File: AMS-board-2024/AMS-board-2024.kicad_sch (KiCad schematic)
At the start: 66 parts, among them J1 XH_6pin_SMT, J10 XH_6pin_SMT, J11 XH_3pin_SMT, J12 XH_4pin_SMT, J13 XH_6pin_SMT, J14 XH_3pin_SMT, J15 XH_4pin_SMT, J16 XH_6pin_SMT, J17 XH_3pin_SMT, J18 XH_4pin_SMT, J19 19427-0040, J2 XH_3pin_SMT, J20 19427-0040, J21 XH_6pin_SMT, J22 XH_3pin_SMT, J23 XH_4pin_SMT, J24 XH_6pin_SMT, J25 XH_3pin_SMT, J26 XH_4pin_SMT, J27 XH_2pin_Side, J28 XH_6pin_Side, J29 XH_5pin_Side, J3 XH_4pin_SMT, J30 PinHeader_02x05_P1.00mm, J31 XH_2pin_Side, J32 5077CR-16-SMC2-BK-TR, J33 XH_5pin_Side, J34 XH_6pin_SMT, J35 XH_6pin_SMT, J36 XH_6pin_SMT, J37 XH_6pin_SMT, J38 XH_6pin_SMT, J39 XH_6pin_SMT, J4 XH_6pin_SMT, J40 XH_6pin_SMT, J41 XH_6pin_SMT, J5 XH_3pin_SMT, J6 XH_4pin_SMT, J7 XH_6pin_SMT, J8 XH_3pin_SMT, J9 XH_4pin_SMT

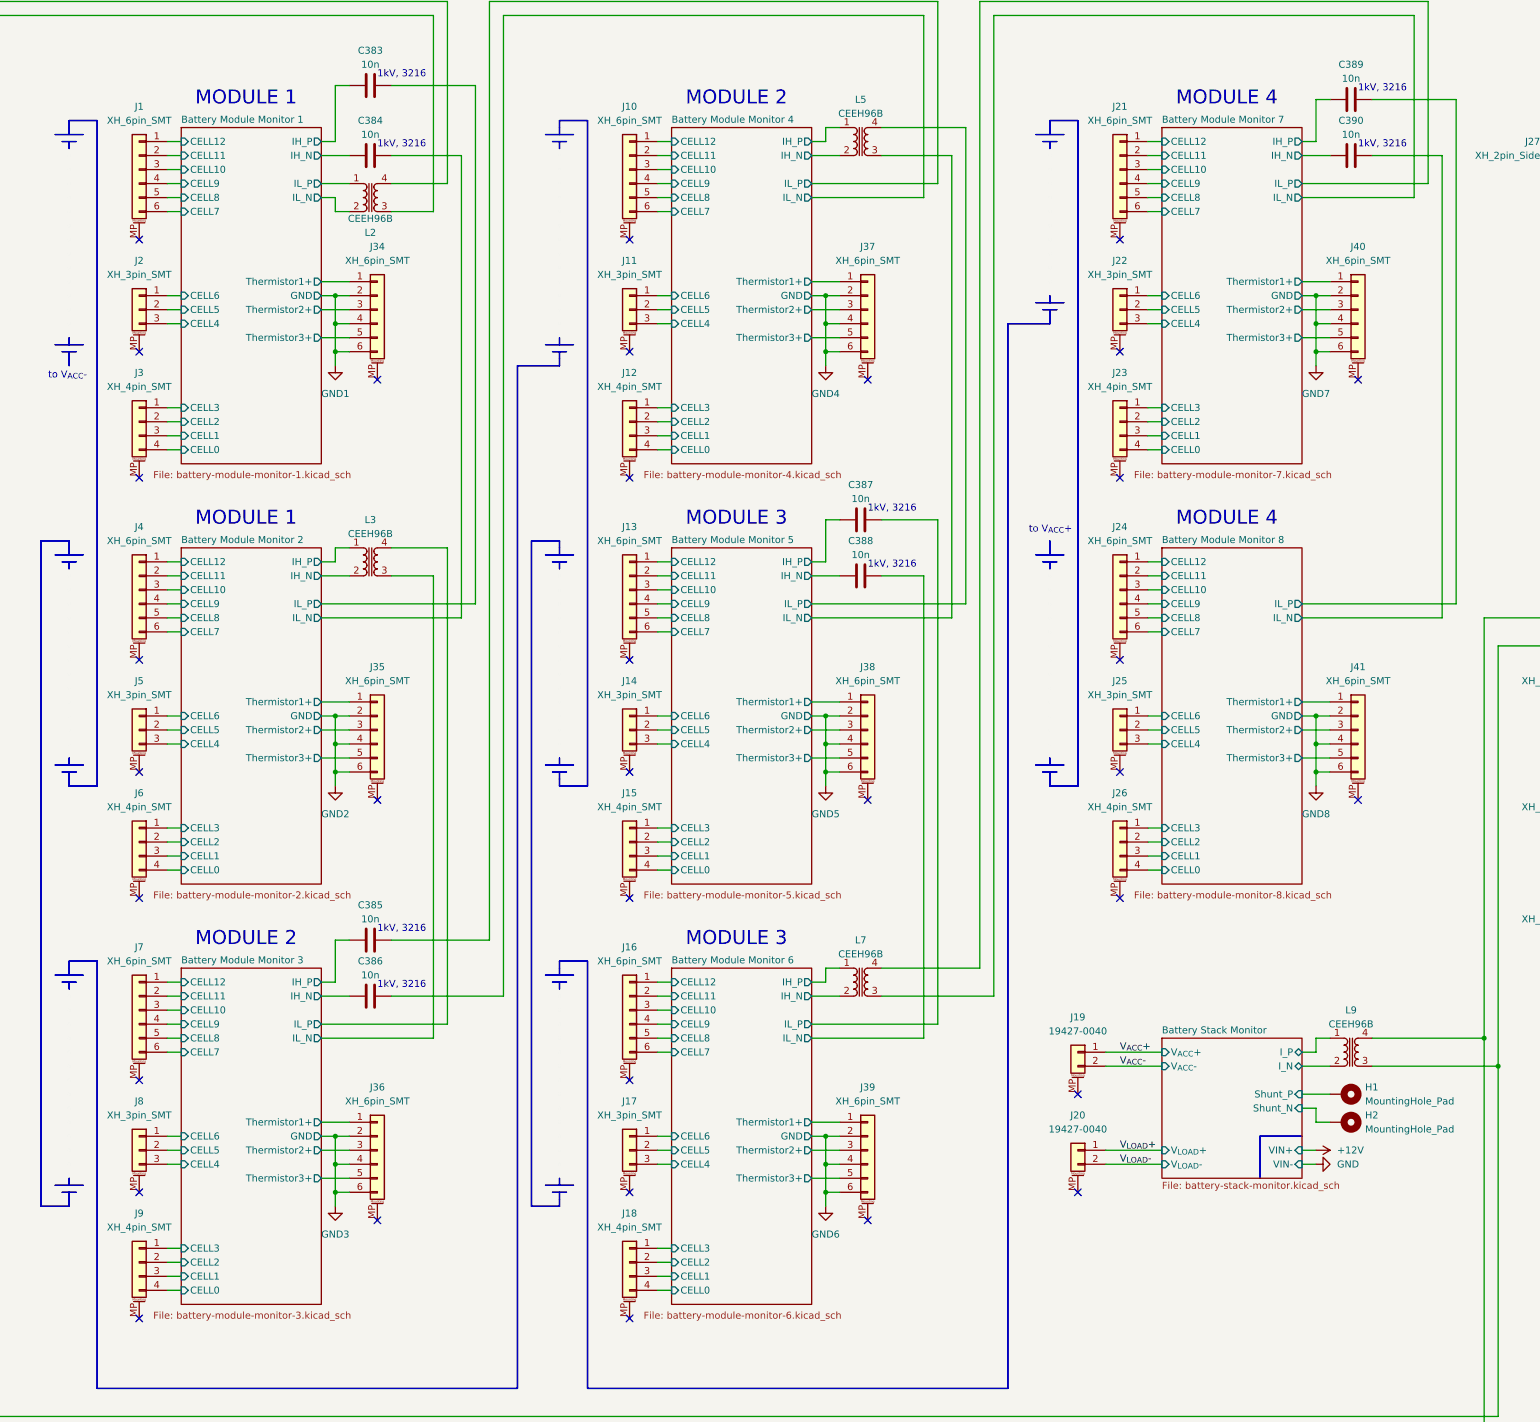
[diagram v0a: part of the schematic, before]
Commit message: セル監視コネクタを34691-0200に変更
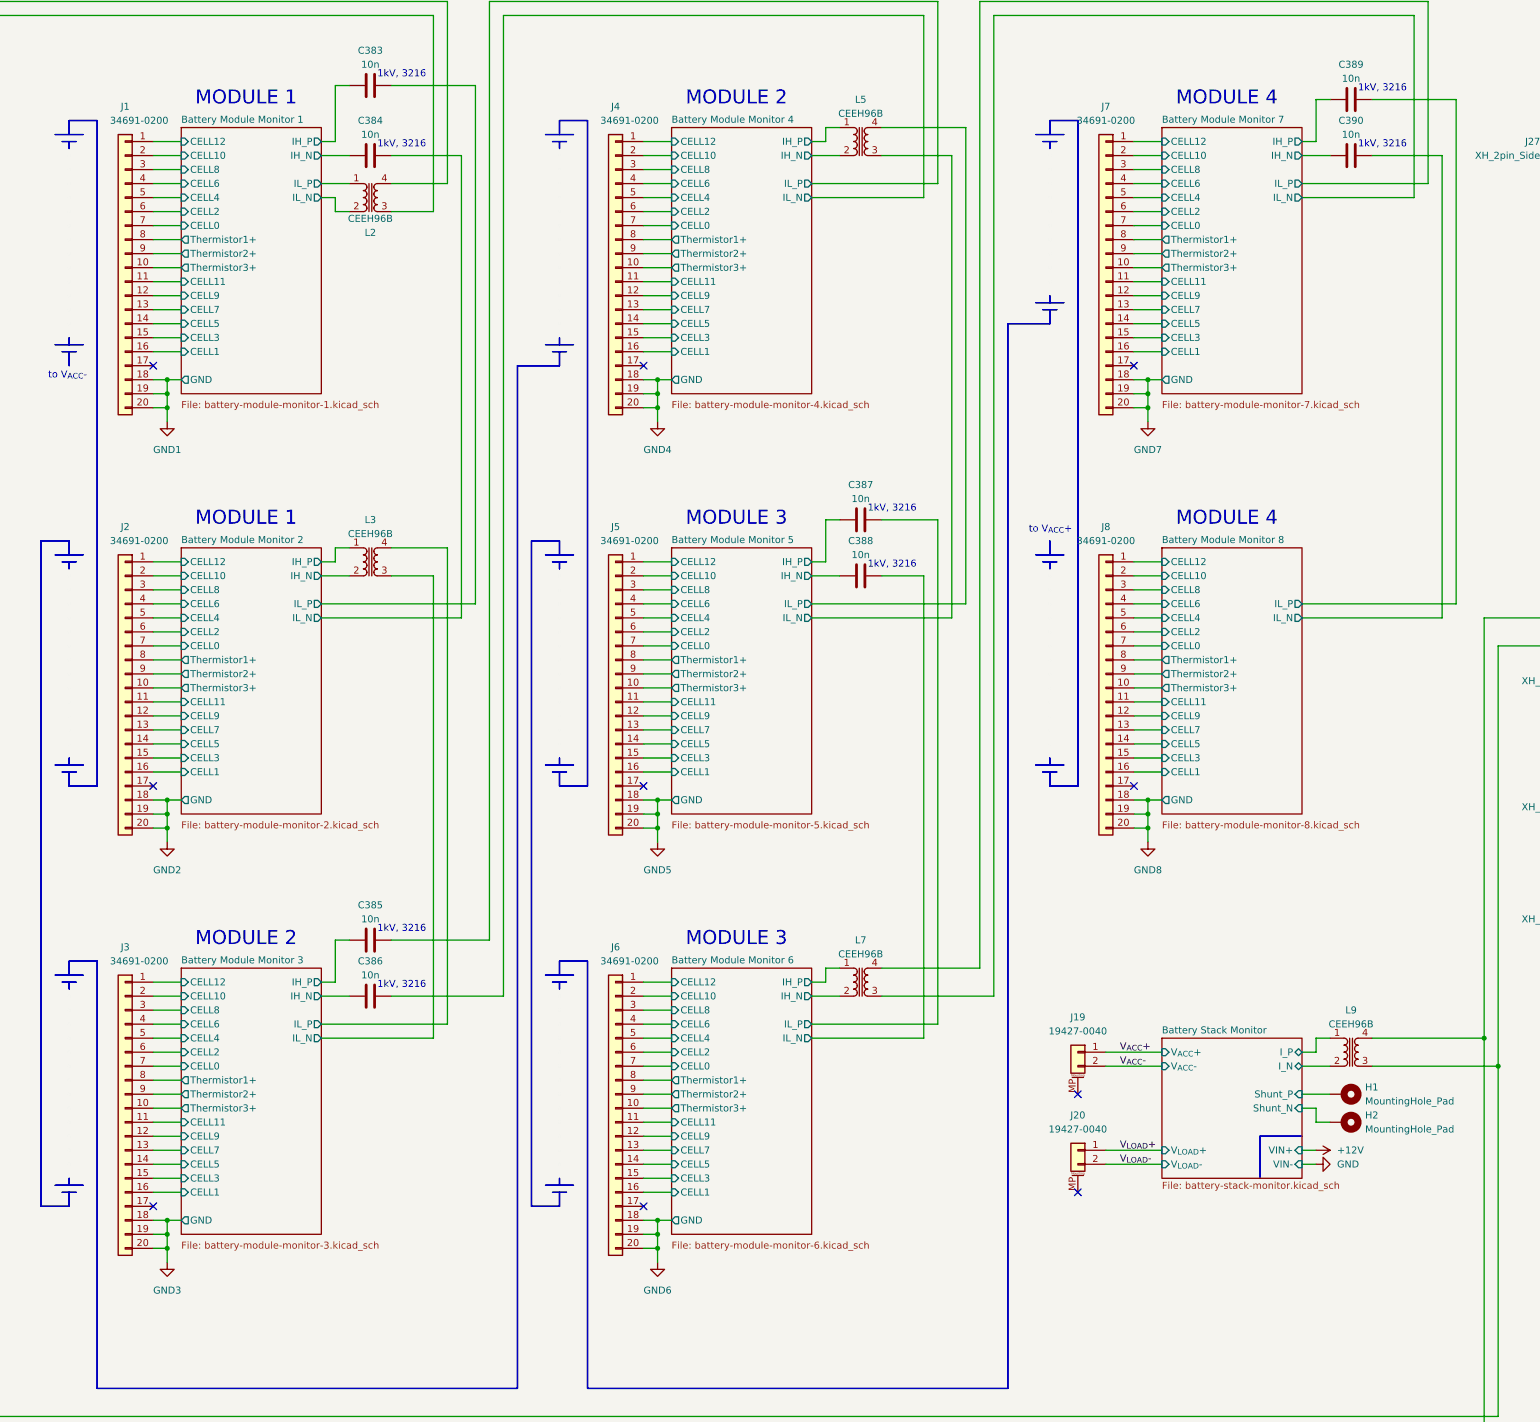
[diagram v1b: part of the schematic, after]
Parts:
- removed J1, J10, J13, J16, J21, J24, J34, J35, J36, J37, J38, J39, J4, J40, J41, J7: XH_6pin_SMT, ProjectEV:Connector_S6B-XH-SM4-TB, symbol ProjectEV:Connector_XH_6pin_SMT
- removed J11, J14, J17, J2, J22, J25, J5, J8: XH_3pin_SMT, ProjectEV:Connector_S3B-XH-SM4-TB, symbol ProjectEV:Connector_XH_3pin_SMT
- removed J12, J15, J18, J23, J26, J3, J6, J9: XH_4pin_SMT, ProjectEV:Connector_S4B-XH-SM4-TB, symbol ProjectEV:Connector_XH_4pin_SMT
- added J1, J2, J3, J4, J5, J6, J7, J8: 34691-0200, ProjectEV:Connector_34691-0200, symbol ProjectEV:Connector_34691-0200
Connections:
- net Battery Module Monitor 1/CELL0: now also J1.7 (Pin_7)
- net Battery Module Monitor 1/CELL1: now also J1.16 (Pin_16)
- net Battery Module Monitor 1/CELL10: now also J1.2 (Pin_2)
- net Battery Module Monitor 1/CELL11: now also J1.11 (Pin_11)
- net Battery Module Monitor 1/CELL12: now also J1.1 (Pin_1)
- net Battery Module Monitor 1/CELL2: now also J1.6 (Pin_6)
- net Battery Module Monitor 1/CELL3: now also J1.15 (Pin_15)
- net Battery Module Monitor 1/CELL4: now also J1.5 (Pin_5)
- net Battery Module Monitor 1/CELL5: now also J1.14 (Pin_14)
- net Battery Module Monitor 1/CELL6: now also J1.4 (Pin_4)
- net Battery Module Monitor 1/CELL7: now also J1.13 (Pin_13)
- net Battery Module Monitor 1/CELL8: now also J1.3 (Pin_3)
- net Battery Module Monitor 1/CELL9: now also J1.12 (Pin_12)
- net Battery Module Monitor 1/Thermistor1+: now also J1.8 (Pin_8)
- net Battery Module Monitor 1/Thermistor2+: now also J1.9 (Pin_9)
- net Battery Module Monitor 1/Thermistor3+: now also J1.10 (Pin_10)
- net Battery Module Monitor 2/CELL0: now also J2.7 (Pin_7)
- net Battery Module Monitor 2/CELL1: now also J2.16 (Pin_16)
- net Battery Module Monitor 2/CELL10: now also J2.2 (Pin_2)
- net Battery Module Monitor 2/CELL11: now also J2.11 (Pin_11)
- net Battery Module Monitor 2/CELL12: now also J2.1 (Pin_1)
- net Battery Module Monitor 2/CELL2: now also J2.6 (Pin_6)
- net Battery Module Monitor 2/CELL3: now also J2.15 (Pin_15)
- net Battery Module Monitor 2/CELL4: now also J2.5 (Pin_5)
- net Battery Module Monitor 2/CELL5: now also J2.14 (Pin_14)
- net Battery Module Monitor 2/CELL6: now also J2.4 (Pin_4)
- net Battery Module Monitor 2/CELL7: now also J2.13 (Pin_13)
- net Battery Module Monitor 2/CELL8: now also J2.3 (Pin_3)
- net Battery Module Monitor 2/CELL9: now also J2.12 (Pin_12)
- net Battery Module Monitor 2/Thermistor1+: now also J2.8 (Pin_8)
- net Battery Module Monitor 2/Thermistor2+: now also J2.9 (Pin_9)
- net Battery Module Monitor 2/Thermistor3+: now also J2.10 (Pin_10)
- net Battery Module Monitor 3/CELL0: now also J3.7 (Pin_7)
- net Battery Module Monitor 3/CELL1: now also J3.16 (Pin_16)
- net Battery Module Monitor 3/CELL10: now also J3.2 (Pin_2)
- net Battery Module Monitor 3/CELL11: now also J3.11 (Pin_11)
- net Battery Module Monitor 3/CELL12: now also J3.1 (Pin_1)
- net Battery Module Monitor 3/CELL2: now also J3.6 (Pin_6)
- net Battery Module Monitor 3/CELL3: now also J3.15 (Pin_15)
- net Battery Module Monitor 3/CELL4: now also J3.5 (Pin_5)
- net Battery Module Monitor 3/CELL5: now also J3.14 (Pin_14)
- net Battery Module Monitor 3/CELL6: now also J3.4 (Pin_4)
- net Battery Module Monitor 3/CELL7: now also J3.13 (Pin_13)
- net Battery Module Monitor 3/CELL8: now also J3.3 (Pin_3)
- net Battery Module Monitor 3/CELL9: now also J3.12 (Pin_12)
- net Battery Module Monitor 3/Thermistor1+: now also J3.8 (Pin_8)
- net Battery Module Monitor 3/Thermistor2+: now also J3.9 (Pin_9)
- net Battery Module Monitor 3/Thermistor3+: now also J3.10 (Pin_10)
- net Battery Module Monitor 4/CELL0: now also J4.7 (Pin_7)
- net Battery Module Monitor 4/CELL1: now also J4.16 (Pin_16)
- net Battery Module Monitor 4/CELL10: now also J4.2 (Pin_2)
- net Battery Module Monitor 4/CELL11: now also J4.11 (Pin_11)
- net Battery Module Monitor 4/CELL12: now also J4.1 (Pin_1)
- net Battery Module Monitor 4/CELL2: now also J4.6 (Pin_6)
- net Battery Module Monitor 4/CELL3: now also J4.15 (Pin_15)
- net Battery Module Monitor 4/CELL4: now also J4.5 (Pin_5)
- net Battery Module Monitor 4/CELL5: now also J4.14 (Pin_14)
- net Battery Module Monitor 4/CELL6: now also J4.4 (Pin_4)
- net Battery Module Monitor 4/CELL7: now also J4.13 (Pin_13)
- net Battery Module Monitor 4/CELL8: now also J4.3 (Pin_3)
- net Battery Module Monitor 4/CELL9: now also J4.12 (Pin_12)
- net Battery Module Monitor 4/Thermistor1+: now also J4.8 (Pin_8)
- net Battery Module Monitor 4/Thermistor2+: now also J4.9 (Pin_9)
- net Battery Module Monitor 4/Thermistor3+: now also J4.10 (Pin_10)
- net Battery Module Monitor 5/CELL0: now also J5.7 (Pin_7)
- net Battery Module Monitor 5/CELL1: now also J5.16 (Pin_16)
- net Battery Module Monitor 5/CELL10: now also J5.2 (Pin_2)
- net Battery Module Monitor 5/CELL11: now also J5.11 (Pin_11)
- net Battery Module Monitor 5/CELL12: now also J5.1 (Pin_1)
- net Battery Module Monitor 5/CELL2: now also J5.6 (Pin_6)
- net Battery Module Monitor 5/CELL3: now also J5.15 (Pin_15)
- net Battery Module Monitor 5/CELL4: now also J5.5 (Pin_5)
- net Battery Module Monitor 5/CELL5: now also J5.14 (Pin_14)
- net Battery Module Monitor 5/CELL6: now also J5.4 (Pin_4)
- net Battery Module Monitor 5/CELL7: now also J5.13 (Pin_13)
- net Battery Module Monitor 5/CELL8: now also J5.3 (Pin_3)
- net Battery Module Monitor 5/CELL9: now also J5.12 (Pin_12)
- net Battery Module Monitor 5/Thermistor1+: now also J5.8 (Pin_8)
- net Battery Module Monitor 5/Thermistor2+: now also J5.9 (Pin_9)
- net Battery Module Monitor 5/Thermistor3+: now also J5.10 (Pin_10)
- net Battery Module Monitor 6/CELL0: now also J6.7 (Pin_7)
- net Battery Module Monitor 6/CELL1: now also J6.16 (Pin_16)
- net Battery Module Monitor 6/CELL10: now also J6.2 (Pin_2)
- net Battery Module Monitor 6/CELL11: now also J6.11 (Pin_11)
- net Battery Module Monitor 6/CELL12: now also J6.1 (Pin_1)
- net Battery Module Monitor 6/CELL2: now also J6.6 (Pin_6)
- net Battery Module Monitor 6/CELL3: now also J6.15 (Pin_15)
- net Battery Module Monitor 6/CELL4: now also J6.5 (Pin_5)
- net Battery Module Monitor 6/CELL5: now also J6.14 (Pin_14)
- net Battery Module Monitor 6/CELL6: now also J6.4 (Pin_4)
- net Battery Module Monitor 6/CELL7: now also J6.13 (Pin_13)
- net Battery Module Monitor 6/CELL8: now also J6.3 (Pin_3)
- net Battery Module Monitor 6/CELL9: now also J6.12 (Pin_12)
- net Battery Module Monitor 6/Thermistor1+: now also J6.8 (Pin_8)
- net Battery Module Monitor 6/Thermistor2+: now also J6.9 (Pin_9)
- net Battery Module Monitor 6/Thermistor3+: now also J6.10 (Pin_10)
- net Battery Module Monitor 7/CELL0: now also J7.7 (Pin_7)
- net Battery Module Monitor 7/CELL1: now also J7.16 (Pin_16)
- net Battery Module Monitor 7/CELL10: now also J7.2 (Pin_2)
- net Battery Module Monitor 7/CELL11: now also J7.11 (Pin_11)
- net Battery Module Monitor 7/CELL12: now also J7.1 (Pin_1)
- net Battery Module Monitor 7/CELL2: now also J7.6 (Pin_6)
- net Battery Module Monitor 7/CELL3: now also J7.15 (Pin_15)
- net Battery Module Monitor 7/CELL4: now also J7.5 (Pin_5)
- net Battery Module Monitor 7/CELL5: now also J7.14 (Pin_14)
- net Battery Module Monitor 7/CELL6: now also J7.4 (Pin_4)
- net Battery Module Monitor 7/CELL7: now also J7.13 (Pin_13)
- net Battery Module Monitor 7/CELL8: now also J7.3 (Pin_3)
- net Battery Module Monitor 7/CELL9: now also J7.12 (Pin_12)
- net Battery Module Monitor 7/Thermistor1+: now also J7.8 (Pin_8)
- net Battery Module Monitor 7/Thermistor2+: now also J7.9 (Pin_9)
- net Battery Module Monitor 7/Thermistor3+: now also J7.10 (Pin_10)
- net Battery Module Monitor 8/CELL0: now also J8.7 (Pin_7)
- net Battery Module Monitor 8/CELL1: now also J8.16 (Pin_16)
- net Battery Module Monitor 8/CELL10: now also J8.2 (Pin_2)
- net Battery Module Monitor 8/CELL11: now also J8.11 (Pin_11)
- net Battery Module Monitor 8/CELL12: now also J8.1 (Pin_1)
- net Battery Module Monitor 8/CELL2: now also J8.6 (Pin_6)
- net Battery Module Monitor 8/CELL3: now also J8.15 (Pin_15)
- net Battery Module Monitor 8/CELL4: now also J8.5 (Pin_5)
- net Battery Module Monitor 8/CELL5: now also J8.14 (Pin_14)
- net Battery Module Monitor 8/CELL6: now also J8.4 (Pin_4)
- net Battery Module Monitor 8/CELL7: now also J8.13 (Pin_13)
- net Battery Module Monitor 8/CELL8: now also J8.3 (Pin_3)
- net Battery Module Monitor 8/CELL9: now also J8.12 (Pin_12)
- net Battery Module Monitor 8/Thermistor1+: now also J8.8 (Pin_8)
- net Battery Module Monitor 8/Thermistor2+: now also J8.9 (Pin_9)
- net Battery Module Monitor 8/Thermistor3+: now also J8.10 (Pin_10)
- net GND1: now also J1.18 (Pin_18), J1.19 (Pin_19), J1.20 (Pin_20)
- net GND2: now also J2.18 (Pin_18), J2.19 (Pin_19), J2.20 (Pin_20)
- net GND3: now also J3.18 (Pin_18), J3.19 (Pin_19), J3.20 (Pin_20)
- net GND4: now also J4.18 (Pin_18), J4.19 (Pin_19), J4.20 (Pin_20)
- net GND5: now also J5.18 (Pin_18), J5.19 (Pin_19), J5.20 (Pin_20)
- net GND6: now also J6.18 (Pin_18), J6.19 (Pin_19), J6.20 (Pin_20)
- net GND7: now also J7.18 (Pin_18), J7.19 (Pin_19), J7.20 (Pin_20)
- net GND8: now also J8.18 (Pin_18), J8.19 (Pin_19), J8.20 (Pin_20)
- no-connect marks 42 -> 18
